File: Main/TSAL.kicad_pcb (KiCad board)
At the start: 2 copper layers, 140 x 70 mm, 81 parts, among them J1 Mini-SPOX, J2 Mini-SPOX, J3 Mini-Fit_Jr, J4 Mini-SPOX, J5 Mini-SPOX, J6 Jumper, J7 Jumper, Q1 IRLML2502, Q2 IRLML2502, Q3 IRLML2502, Q4 IRLML2502, Q5 IRF8721, U1 74HC08, U2 74HC08, U3 TLV70033, U4 LMC555, U5 LMR14030, U6 ZLDO1117G50, U7 TPS62205, U8 MAX40200AUK

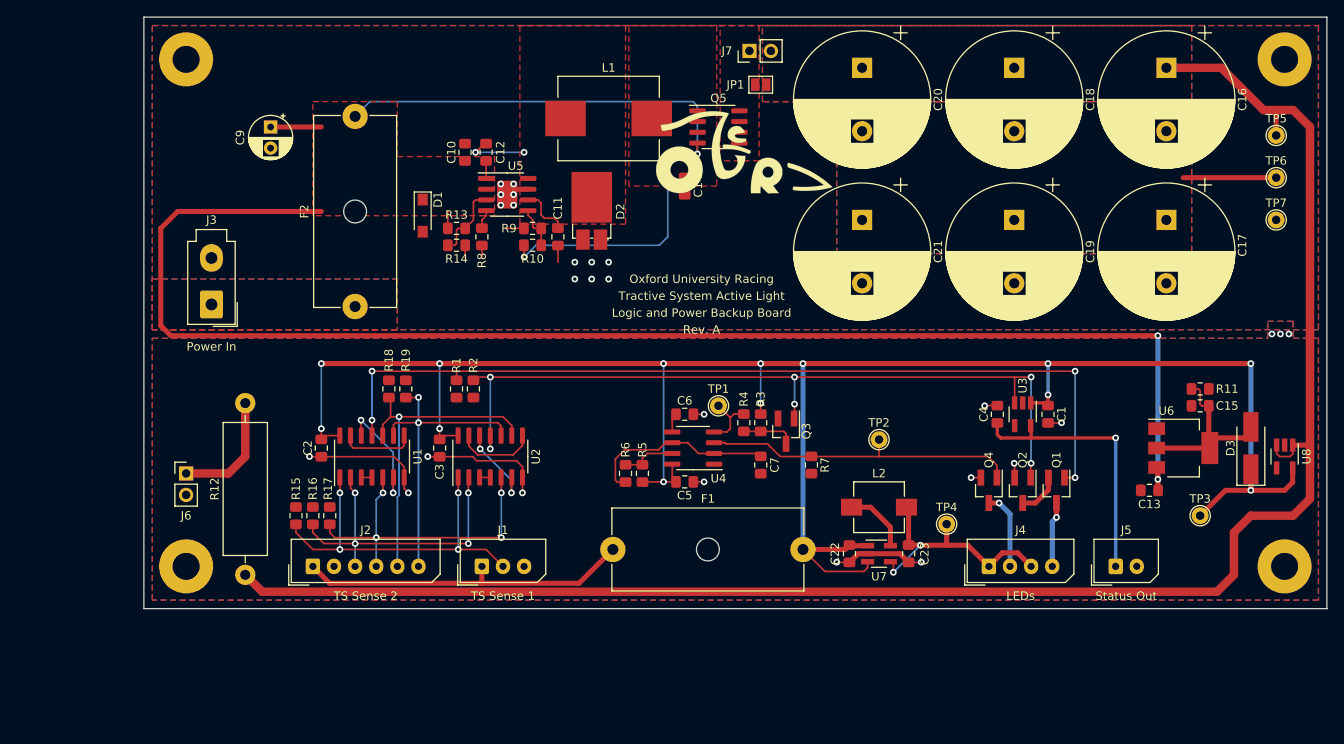
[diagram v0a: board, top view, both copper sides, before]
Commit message: Added first rev of design of new TSAL main board
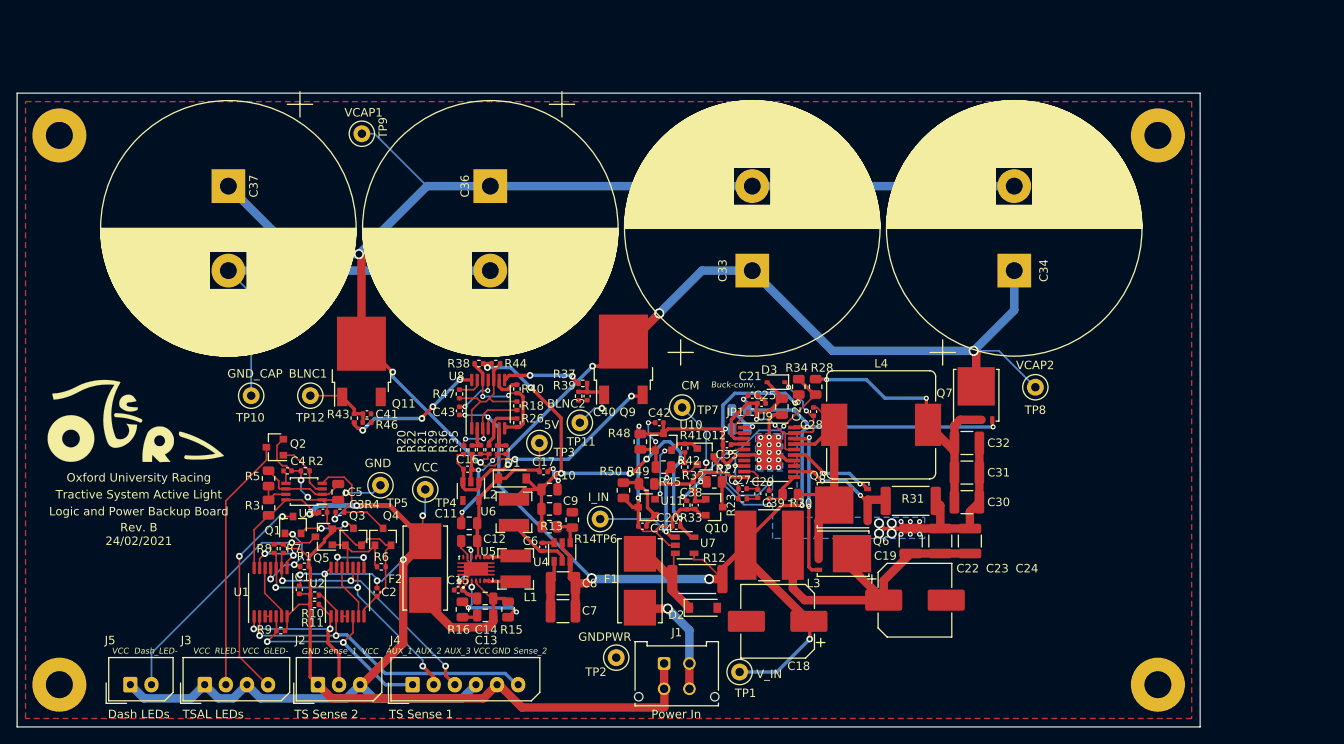
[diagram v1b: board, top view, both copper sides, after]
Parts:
- removed J6, J7: Jumper, Connector_PinHeader_2.54mm:PinHeader_1x02_P2.54mm_Vertical
- added C24: 10uF, Capacitor_SMD:C_1210_3225Metric, F.Cu at (177.8, 122.0)
- added C25: 0.1uF, Capacitor_SMD:C_0402_1005Metric, F.Cu at (153.1, 105.7)
- added C26: 10uF, Capacitor_SMD:C_0805_2012Metric, F.Cu at (155.5, 106.1)
- added C27: 100pF, Capacitor_SMD:C_0402_1005Metric, F.Cu at (150.8, 115.8)
- added C28: 0.1uF, Capacitor_SMD:C_0402_1005Metric, F.Cu at (159.2, 106.7)
- added C29: 1nF, Capacitor_SMD:C_0402_1005Metric, F.Cu at (152.7, 116.4)
- added C30: 100uF, Capacitor_SMD:C_1210_3225Metric, F.Cu at (177.4, 117.4)
- added C31: 100uF, Capacitor_SMD:C_1210_3225Metric, F.Cu at (177.4, 113.9)
- added C32: 100uF, Capacitor_SMD:C_1210_3225Metric, F.Cu at (177.4, 110.4)
- added C33: 200F, Capacitor_THT:CP_Radial_D30.0mm_P10.00mm_SnapIn, F.Cu at (152.0, 90.0)
- added C34: 200F, Capacitor_THT:CP_Radial_D30.0mm_P10.00mm_SnapIn, F.Cu at (183.0, 90.0)
- added C35: 0.1uF, Capacitor_SMD:C_0402_1005Metric, F.Cu at (149.0, 110.6)
- added C36: 200F, Capacitor_THT:CP_Radial_D30.0mm_P10.00mm_SnapIn, F.Cu at (121.0, 80.0)
- added C37: 200F, Capacitor_THT:CP_Radial_D30.0mm_P10.00mm_SnapIn, F.Cu at (90.0, 80.0)
- added C38: 0.1uF, Capacitor_SMD:C_0402_1005Metric, F.Cu at (145.2, 117.8)
- added C39: 1nF, Capacitor_SMD:C_0402_1005Metric, F.Cu at (154.0, 116.5)
- added C40: 0.1uF, Capacitor_SMD:C_0402_1005Metric, F.Cu at (132.4, 104.8)
- added C41: 0.1uF, Capacitor_SMD:C_0402_1005Metric, F.Cu at (106.4, 107.0)
- added C42: 1nF, Capacitor_SMD:C_0402_1005Metric, F.Cu at (141.0, 108.0)
- added C43: 0.1uF, Capacitor_SMD:C_0402_1005Metric, F.Cu at (117.3, 106.6)
- added C44: 1nF, Capacitor_SMD:C_0402_1005Metric, F.Cu at (139.0, 120.2)
- added C8: 10uF, Capacitor_SMD:C_1210_3225Metric, F.Cu at (129.6, 127.0)
- added L3: 2.2uH, Inductor_SMD:L_Bourns-SRN8040_8x8.15mm, F.Cu at (154.0, 122.5)
- added L4: 3.3uH, Inductor_SMD:L_Bourns_SRP1245A, F.Cu at (167.2, 108.2)
- added Q10: NPN, Package_TO_SOT_SMD:SOT-23, F.Cu at (147.5, 118.0)
- added Q11: MJD122, Package_TO_SOT_SMD:TO-252-2, F.Cu at (105.8, 100.8)
- added Q12: PNP, Package_TO_SOT_SMD:SOT-23, F.Cu at (146.5, 112.0)
- added Q6: BSC0904NSI, Package_TO_SOT_SMD:TDSON-8-1, F.Cu at (162.8, 123.5)
- added Q7: BSC0902NSI, Package_TO_SOT_SMD:TDSON-8-1, F.Cu at (178.5, 104.8)
- added Q8: BSC0902NSI, Package_TO_SOT_SMD:TDSON-8-1, F.Cu at (162.8, 117.8)
- added Q9: MJD122, Package_TO_SOT_SMD:TO-252-2, F.Cu at (136.8, 100.5)
- added R20: 10k, Resistor_SMD:R_0402_1005Metric, F.Cu at (117.8, 111.2)
- added R21: 10k, Resistor_SMD:R_0402_1005Metric, F.Cu at (119.8, 111.2)
- added R22: 10k, Resistor_SMD:R_0402_1005Metric, F.Cu at (118.8, 111.2)
- added R23: 47k, Resistor_SMD:R_0402_1005Metric, F.Cu at (150.8, 117.0)
- added R24: 0, project:Trace_0.4mmx0.8mm, F.Cu at (158.0, 109.9)
- added R25: 0, project:Trace_0.4mmx0.8mm, F.Cu at (158.0, 111.8)
- added R26: 10k, Resistor_SMD:R_0402_1005Metric, F.Cu at (124.2, 108.0)
- added R27: 15k, Resistor_SMD:R_0805_2012Metric, F.Cu at (147.5, 115.0)
- added R28: 68k, Resistor_SMD:R_0805_2012Metric, F.Cu at (159.5, 103.8)
- added R29: 10k, Resistor_SMD:R_0402_1005Metric, F.Cu at (120.8, 111.2)
- added R30: 56k, Resistor_SMD:R_0805_2012Metric, F.Cu at (156.5, 116.5)
- added R31: 0.006, Resistor_SMD:R_2512_6332Metric, F.Cu at (170.8, 117.2)
- added R32: 10k, Resistor_SMD:R_0402_1005Metric, F.Cu at (145.0, 115.5)
- added R33: 47k, Resistor_SMD:R_0402_1005Metric, F.Cu at (144.2, 117.8)
- added R34: 12k, Resistor_SMD:R_0805_2012Metric, F.Cu at (157.5, 103.8)
- added R35: 10k, Resistor_SMD:R_0402_1005Metric, F.Cu at (122.8, 111.2)
- added R36: 10k, Resistor_SMD:R_0402_1005Metric, F.Cu at (121.8, 111.2)
- added R37: 1k, Resistor_SMD:R_0402_1005Metric, F.Cu at (131.9, 103.3)
- added R38: 47k, Resistor_SMD:R_0402_1005Metric, F.Cu at (119.7, 101.0)
- added R39: 100k, Resistor_SMD:R_0402_1005Metric, F.Cu at (131.4, 104.8)
- added R40: 1k, Resistor_SMD:R_0402_1005Metric, F.Cu at (124.2, 104.0)
- added R41: 10k, Resistor_SMD:R_0402_1005Metric, F.Cu at (144.0, 111.0)
- added R42: 1k, Resistor_SMD:R_0402_1005Metric, F.Cu at (144.0, 113.2)
- added R43: 1k, Resistor_SMD:R_0402_1005Metric, F.Cu at (104.9, 107.5)
- added R44: 47k, Resistor_SMD:R_0402_1005Metric, F.Cu at (121.7, 101.0)
- added R45: 15k, Resistor_SMD:R_0805_2012Metric, F.Cu at (141.5, 113.2)
- added R46: 100k, Resistor_SMD:R_0402_1005Metric, F.Cu at (106.4, 108.0)
- added R47: 1k, Resistor_SMD:R_0402_1005Metric, F.Cu at (117.3, 104.6)
- added R48: 10k, Resistor_SMD:R_0805_2012Metric, F.Cu at (138.8, 110.2)
- added R49: 10k, Resistor_SMD:R_0805_2012Metric, F.Cu at (139.5, 115.2)
- added R50: 15k, Resistor_SMD:R_0805_2012Metric, F.Cu at (136.8, 116.0)
- added TP10: ~, TestPoint:TestPoint_Loop_D2.50mm_Drill1.0mm, F.Cu at (92.7, 104.8)
- added TP11: ~, TestPoint:TestPoint_Loop_D2.50mm_Drill1.0mm, F.Cu at (131.6, 108.0)
- added TP12: ~, TestPoint:TestPoint_Loop_D2.50mm_Drill1.0mm, F.Cu at (99.7, 104.8)
- added TP8: ~, TestPoint:TestPoint_Loop_D2.50mm_Drill1.0mm, F.Cu at (185.5, 103.8)
- added TP9: ~, TestPoint:TestPoint_Loop_D2.50mm_Drill1.0mm, F.Cu at (105.8, 73.8)
- added U10: TLV431, Package_TO_SOT_SMD:SOT-23, F.Cu at (141.5, 110.2)
- added U11: TLV431, Package_TO_SOT_SMD:SOT-23, F.Cu at (139.5, 118.0)
- added U9: LM25117, Package_SO:ETSSOP-20-1EP_4.4x6.5mm_P0.65mm_EP3x4.2mm, F.Cu at (154.0, 111.5)
- added ZZ1: ~, project:Trace_0.2mmx0.6mm, F.Cu at (142.7, 123.9)
- added ZZ2: ~, project:Trace_0.2mmx0.6mm, F.Cu at (145.1, 124.0)
- added ZZ3: ~, project:Trace_1mmx2mm, F.Cu at (141.6, 140.9)
- added ZZ4: ~, project:Trace_0.2mmx0.6mm, F.Cu at (117.3, 111.8)
- added ZZ5: ~, project:Trace_0.2mmx0.6mm, F.Cu at (157.8, 113.8)
- added ZZ6: ~, project:Trace_0.2mmx0.6mm, F.Cu at (120.7, 112.1)
- added ZZ7: ~, project:Trace_0.2mmx0.6mm, F.Cu at (157.0, 112.8)
- added ZZ8: ~, project:Trace_0.4mmx0.8mm, F.Cu at (152.0, 111.8)
- added ZZ9: ~, project:Trace_0.2mmx0.6mm, F.Cu at (122.3, 111.7)
- C1, C15, C4: value 10u -> 0.1uF; footprint Capacitor_SMD:C_0805_2012Metric_Pad1.15x1.40mm_HandSolder -> Capacitor_SMD:C_0402_1005Metric
- C10, C13, C14: value 10u -> 10uF; footprint Capacitor_SMD:C_0805_2012Metric_Pad1.15x1.40mm_HandSolder -> Capacitor_SMD:C_0805_2012Metric
- C11, C12: value 100n -> 10uF; footprint Capacitor_SMD:C_0805_2012Metric_Pad1.15x1.40mm_HandSolder -> Capacitor_SMD:C_0805_2012Metric
- C16, C17: value 35 -> 0.1uF; footprint Capacitor_THT:CP_Radial_D16.0mm_P7.50mm -> Capacitor_SMD:C_0402_1005Metric
- C18, C19: value 35 -> 220uF; footprint Capacitor_THT:CP_Radial_D16.0mm_P7.50mm -> Capacitor_SMD:CP_Elec_8x10.5
- C2, C3, C6: value 100n -> 0.1uF; footprint Capacitor_SMD:C_0805_2012Metric_Pad1.15x1.40mm_HandSolder -> Capacitor_SMD:C_0402_1005Metric
- C20, C21: value DNP -> 0.1uF; footprint Capacitor_THT:CP_Radial_D16.0mm_P7.50mm -> Capacitor_SMD:C_0402_1005Metric
- C22, C23: value 10u -> 10uF; footprint Capacitor_SMD:C_0805_2012Metric_Pad1.15x1.40mm_HandSolder -> Capacitor_SMD:C_1210_3225Metric
- C5: value 100n -> 2.2uF; footprint Capacitor_SMD:C_0805_2012Metric_Pad1.15x1.40mm_HandSolder -> Capacitor_SMD:C_0805_2012Metric
- C7: value 2.2u -> 10uF; footprint Capacitor_SMD:C_0805_2012Metric_Pad1.15x1.40mm_HandSolder -> Capacitor_SMD:C_1210_3225Metric
- C9: value 100u -> 10uF; footprint Capacitor_THT:CP_Radial_D5.0mm_P2.50mm -> Capacitor_SMD:C_0805_2012Metric
- D1: value SMF4L15A -> ~; footprint project:D_SOD-123_HandSolder -> Diode_SMD:D_SOD-123
- D2: value FSV1045V -> SMF4L15A; footprint project:TO-277A_HandSolder -> Diode_SMD:D_SOD-123
- D3: value S1A -> ~; footprint Diode_SMD:D_SMA_Handsoldering -> Diode_SMD:D_SOD-323
- F1: value 1A -> 6A; footprint Fuse:Fuseholder_Cylinder-5x20mm_Schurter_0031_8201_Horizontal_Open -> footprints_archive_old_design:Fuseholder_Littelfuse_Nano2_154x
- F2: value 3A -> 1A; footprint Fuse:Fuseholder_Cylinder-5x20mm_Schurter_0031_8201_Horizontal_Open -> footprints_archive_old_design:Fuseholder_Littelfuse_Nano2_154x
- J1: value Mini-SPOX -> Micro-Fit; footprint Connector_Molex:Molex_SPOX_5267-03A_1x03_P2.50mm_Vertical -> Connector_Molex:Molex_Micro-Fit_3.0_43045-0412_2x02_P3.00mm_Vertical
- J2: footprint Connector_Molex:Molex_SPOX_5267-06A_1x06_P2.50mm_Vertical -> Connector_Molex:Molex_SPOX_5267-03A_1x03_P2.50mm_Vertical
- J3: value Mini-Fit_Jr -> Mini-SPOX; footprint Connector_Molex:Molex_Mini-Fit_Jr_5566-02A_2x01_P4.20mm_Vertical -> Connector_Molex:Molex_SPOX_5267-04A_1x04_P2.50mm_Vertical
- J4: footprint Connector_Molex:Molex_SPOX_5267-04A_1x04_P2.50mm_Vertical -> Connector_Molex:Molex_SPOX_5267-06A_1x06_P2.50mm_Vertical
- JP1: value Jumper -> 0; footprint Jumper:SolderJumper-2_P1.3mm_Open_Pad1.0x1.5mm -> Resistor_SMD:R_0402_1005Metric
- L1: value 15u -> 1.5uH; footprint project:104CDMCCDS -> Inductor_SMD:L_Bourns-SRN4018
- L2: value 10u -> 4.7uH; footprint project:CDRH62B -> Inductor_SMD:L_Bourns-SRN4018
- Q1, Q2, Q3, Q4: footprint Package_TO_SOT_SMD:SOT-23_Handsoldering -> Package_TO_SOT_SMD:SOT-23
- Q5: value IRF8721 -> IRLML2502; footprint Package_SO:SOIC-8_3.9x4.9mm_P1.27mm -> Package_TO_SOT_SMD:SOT-23
- R1, R2, R6, R7, R8: footprint Resistor_SMD:R_0805_2012Metric_Pad1.15x1.40mm_HandSolder -> Resistor_SMD:R_0402_1005Metric
- R10: value 130k -> 100k; footprint Resistor_SMD:R_0805_2012Metric_Pad1.15x1.40mm_HandSolder -> Resistor_SMD:R_0402_1005Metric
- R11: value 1k -> 100k; footprint Resistor_SMD:R_0805_2012Metric_Pad1.15x1.40mm_HandSolder -> Resistor_SMD:R_0402_1005Metric
- R12: value 4.7 -> 0.006; footprint Resistor_THT:R_Axial_DIN0516_L15.5mm_D5.0mm_P20.32mm_Horizontal -> Resistor_SMD:R_2512_6332Metric
- R13: value 820k -> 56k; footprint Resistor_SMD:R_0805_2012Metric_Pad1.15x1.40mm_HandSolder -> Resistor_SMD:R_0805_2012Metric
- R14, R16: value 100k -> 10k; footprint Resistor_SMD:R_0805_2012Metric_Pad1.15x1.40mm_HandSolder -> Resistor_SMD:R_0805_2012Metric
- R15: value 100k -> 56k; footprint Resistor_SMD:R_0805_2012Metric_Pad1.15x1.40mm_HandSolder -> Resistor_SMD:R_0805_2012Metric
- R17: value 100k -> 68k; footprint Resistor_SMD:R_0805_2012Metric_Pad1.15x1.40mm_HandSolder -> Resistor_SMD:R_0805_2012Metric; moved to B.Cu
- R18: value 100k -> 10k; footprint Resistor_SMD:R_0805_2012Metric_Pad1.15x1.40mm_HandSolder -> Resistor_SMD:R_0402_1005Metric
- R19: value 100k -> 10k; footprint Resistor_SMD:R_0805_2012Metric_Pad1.15x1.40mm_HandSolder -> Resistor_SMD:R_0805_2012Metric; moved to B.Cu
- R3: value 22k -> 10k; footprint Resistor_SMD:R_0805_2012Metric_Pad1.15x1.40mm_HandSolder -> Resistor_SMD:R_0805_2012Metric
- R4: value 1k -> 10k; footprint Resistor_SMD:R_0805_2012Metric_Pad1.15x1.40mm_HandSolder -> Resistor_SMD:R_0402_1005Metric
- R5: value 22k -> 100k; footprint Resistor_SMD:R_0805_2012Metric_Pad1.15x1.40mm_HandSolder -> Resistor_SMD:R_0805_2012Metric
- R9: value 22k -> 100k; footprint Resistor_SMD:R_0805_2012Metric_Pad1.15x1.40mm_HandSolder -> Resistor_SMD:R_0402_1005Metric
- TP1: value TP_Timer_En -> ~; footprint TestPoint:TestPoint_THTPad_D2.0mm_Drill1.0mm -> TestPoint:TestPoint_Loop_D2.50mm_Drill1.0mm
- TP2: value TP_RLED_Ctrl -> ~; footprint TestPoint:TestPoint_THTPad_D2.0mm_Drill1.0mm -> TestPoint:TestPoint_Loop_D2.50mm_Drill1.0mm
- TP3: value TP_VCC -> ~; footprint TestPoint:TestPoint_THTPad_D2.0mm_Drill1.0mm -> TestPoint:TestPoint_Loop_D2.50mm_Drill1.0mm
- TP4: value TP_2V5 -> ~; footprint TestPoint:TestPoint_THTPad_D2.0mm_Drill1.0mm -> TestPoint:TestPoint_Loop_D2.50mm_Drill1.0mm
- TP5: value TP_Vcap -> ~; footprint TestPoint:TestPoint_THTPad_D2.0mm_Drill1.0mm -> TestPoint:TestPoint_Loop_D2.50mm_Drill1.0mm
- TP6: value TP_Vmid -> ~; footprint TestPoint:TestPoint_THTPad_D2.0mm_Drill1.0mm -> TestPoint:TestPoint_Loop_D2.50mm_Drill1.0mm
- TP7: value TP_GND -> ~; footprint TestPoint:TestPoint_THTPad_D2.0mm_Drill1.0mm -> TestPoint:TestPoint_Loop_D2.50mm_Drill1.0mm
- U1, U2: footprint Package_SO:SOIC-14_3.9x8.7mm_P1.27mm -> Package_SO:TSSOP-14_4.4x5mm_P0.65mm
- U3: value TLV70033 -> LMC555; footprint Package_TO_SOT_SMD:SOT-23-5_HandSoldering -> Package_SO:TSSOP-8_3x3mm_P0.65mm
- U4: value LMC555 -> TPS562200; footprint Package_SO:SOIC-8_3.9x4.9mm_P1.27mm -> Package_TO_SOT_SMD:SOT-23-6
- U5: value LMR14030 -> TPS63020; footprint Package_SO:SOIC-8-1EP_3.9x4.9mm_P1.27mm_EP2.41x3.3mm -> project:TPS63020
- U6: value ZLDO1117G50 -> MAX40200AUK; footprint Package_TO_SOT_SMD:SOT-223-3_TabPin2 -> Package_TO_SOT_SMD:SOT-23-5
- U7: value TPS62205 -> INA180A3; footprint Package_TO_SOT_SMD:SOT-23-5_HandSoldering -> Package_TO_SOT_SMD:SOT-23-5
- U8: value MAX40200AUK -> TLV9104; footprint Package_TO_SOT_SMD:SOT-23-5_HandSoldering -> Package_SO:TSSOP-14_4.4x5mm_P0.65mm
- moved J5 117.4 mm to (78.4, 139.0)
- moved TP5 113.8 mm to (108.0, 115.4), turned to 90 degrees
- moved R11 107.9 mm to (100.2, 129.5), turned to 180 degrees
- moved C16 95.4 mm to (118.3, 113.5), turned to 0 degrees
- moved U8 94.5 mm to (120.8, 105.8), turned to 90 degrees
- moved C1 91.0 mm to (98.4, 127.8)
- moved C15 90.5 mm to (117.2, 127.8), turned to 0 degrees
- moved Q1 90.4 mm to (97.7, 120.1), turned to 90 degrees
- moved TP6 89.6 mm to (134.0, 119.4), turned to 90 degrees
- moved Q2 88.6 mm to (95.5, 110.9), turned to 180 degrees
- moved U3 85.5 mm to (99.0, 116.1), turned to 180 degrees
- moved U6 84.5 mm to (118.7, 116.1), turned to 270 degrees
- moved C4 84.3 mm to (97.0, 113.7), turned to 0 degrees
- moved C13 80.0 mm to (120.4, 130.8)
- moved C17 79.5 mm to (127.3, 113.8), turned to 0 degrees
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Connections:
- C10 pad 1: /Power/VIN_F -> +5V
- C10 pad 2: GND -> GNDPWR
- C11 pad 2: GND -> GNDPWR
- C12 pad 1: Net-(C12-Pad1) -> Net-(C11-Pad1)
- C12 pad 2: Net-(C12-Pad2) -> GNDPWR
- C13 pad 1: /Power/VIN_F -> Net-(C13-Pad1)
- C13 pad 2: GND -> GNDPWR
- C14 pad 1: Net-(C14-Pad1) -> Net-(C13-Pad1)
- C14 pad 2: GND -> GNDPWR
- C15 pad 2: GND -> GNDPWR
- C16 pad 1: /Power/Vcap -> /Power/VCAP2
- C16 pad 2: Net-(C16-Pad2) -> GNDPWR
- C17 pad 1: Net-(C16-Pad2) -> Net-(C11-Pad1)
- C17 pad 2: GND -> GNDPWR
- C18 pad 1: /Power/Vcap -> /Power/V_IN
- C18 pad 2: Net-(C16-Pad2) -> GNDPWR
- C19 pad 1: Net-(C16-Pad2) -> Net-(C19-Pad1)
- C19 pad 2: GND -> GNDPWR
- C20 pad 1: /Power/Vcap -> +5V
- C20 pad 2: Net-(C16-Pad2) -> GNDA
- C21 pad 1: Net-(C16-Pad2) -> /Power/V_IN
- C21 pad 2: GND -> GNDPWR
- C22 pad 1: VCC -> Net-(C19-Pad1)
- C22 pad 2: GND -> GNDPWR
- C23 pad 1: +2V5 -> Net-(C19-Pad1)
- C23 pad 2: GND -> GNDPWR
- C4 pad 1: /TS_Inact_Out -> Net-(C4-Pad1)
- C5 pad 1: VCC -> Net-(C5-Pad1)
- C6 pad 2: GND -> Net-(C6-Pad2)
- C7 pad 1: Net-(C7-Pad1) -> /Power/V_IN
- C7 pad 2: GND -> GNDPWR
- C9 pad 1: /Power/VIN_F -> +5V
- C9 pad 2: GND -> GNDPWR
- D1 pad 1: /Power/VIN_F -> Net-(C11-Pad1)
- D1 pad 2: GND -> +5V
- D2 pad 1: GND -> Net-(D2-Pad1)
- D2 pad 2: GND -> GNDPWR
- D3 pad 1: VCC -> /Power/HB
- D3 pad 2: Net-(C15-Pad1) -> /Power/BUCK_VCC
- F1 pad 1: /VCC_F -> Net-(D2-Pad1)
- F1 pad 2: VCC -> VIN
- F2 pad 1: /Power/VIN_F -> VCC
- F2 pad 2: VIN -> Net-(C13-Pad1)
- J1 pad 1: /VCC_F -> GNDPWR
- J1 pad 2: /Sense_1 -> VIN
- J1 pad 3: GND -> GNDPWR
- J2 pad 1: /VCC_F -> GND
- J2 pad 2: GND -> /Sense_1
- J2 pad 3: /Sense_2 -> VCC
- J3 pad 1: VIN -> VCC
- J3 pad 2: GND -> /RLED-
- J4 pad 1: +2V5 -> /AUX_1
- J4 pad 2: /RLED- -> /AUX_2
- J4 pad 3: +2V5 -> /AUX_3
- J4 pad 4: /GLED- -> VCC
- J5 pad 1: /TS_Inact_Out -> VCC
- J5 pad 2: GND -> /Dash_LED-
- JP1 pad 1: Net-(J7-Pad1) -> /Power/BUCK_VCC
- JP1 pad 2: /Power/Vcap -> /Power/DEMB
- L1 pad 1: Net-(C12-Pad2) -> Net-(L1-Pad1)
- L1 pad 2: Net-(C14-Pad1) -> Net-(L1-Pad2)
- L2 pad 1: Net-(L2-Pad1) -> Net-(C6-Pad1)
- L2 pad 2: +2V5 -> +5V
- Q2 pad 3: Net-(Q1-Pad2) -> /RLED-
- Q3 pad 1: Net-(Q2-Pad1) -> Net-(Q3-Pad1)
- Q3 pad 3: Net-(Q3-Pad3) -> Net-(Q1-Pad2)
- Q4 pad 1: Net-(Q4-Pad1) -> Net-(Q3-Pad1)
- Q4 pad 3: /RLED- -> Net-(Q4-Pad3)
- Q5 pad 1: Net-(C14-Pad1) -> Net-(Q3-Pad1)
- Q5 pad 2: Net-(C14-Pad1) -> GND
- Q5 pad 3: Net-(C14-Pad1) -> /Dash_LED-
- R10 pad 1: Net-(C14-Pad1) -> /Sense_2
- R10 pad 2: Net-(R10-Pad2) -> GND
- R11 pad 1: Net-(C15-Pad1) -> /Sense_1
- R12 pad 1: /Power/Vcap -> Net-(D2-Pad1)
- R12 pad 2: Net-(J6-Pad1) -> /Power/V_IN
- R13 pad 1: /Power/VIN_F -> +5V
- R14 pad 2: GND -> GNDPWR
- R15 pad 1: /Sense_1 -> Net-(C13-Pad1)
- R15 pad 2: GND -> Net-(R15-Pad2)
- R16 pad 1: /Sense_2 -> Net-(R15-Pad2)
- R16 pad 2: GND -> GNDPWR
- R17 pad 1: /AUX_1 -> /Power/V_IN
- R17 pad 2: GND -> /Power/UVLO
- R18 pad 1: /AUX_2 -> Net-(R18-Pad1)
- R18 pad 2: GND -> /Power/CAP_D2
- R19 pad 1: /AUX_3 -> /Power/UVLO
- R19 pad 2: GND -> GNDA
- R3 pad 2: Net-(Q3-Pad3) -> Net-(R3-Pad2)
- R4 pad 1: Net-(R4-Pad1) -> VCC
- R4 pad 2: Net-(Q3-Pad3) -> Net-(Q4-Pad3)
- R5 pad 1: VCC -> Net-(R3-Pad2)
- R5 pad 2: Net-(R5-Pad2) -> Net-(C5-Pad1)
- R6 pad 1: Net-(R5-Pad2) -> Net-(Q3-Pad1)
- R6 pad 2: Net-(C7-Pad1) -> GND
- R7 pad 1: Net-(Q4-Pad1) -> /AUX_3
- R8 pad 1: Net-(R8-Pad1) -> /AUX_2
- R9 pad 1: Net-(R10-Pad2) -> /AUX_1
- TP1 pad 1: Net-(R4-Pad1) -> /Power/V_IN
- TP2 pad 1: Net-(Q4-Pad1) -> GNDPWR
- TP3 pad 1: VCC -> Net-(C11-Pad1)
- TP4 pad 1: +2V5 -> VCC
- TP5 pad 1: /Power/Vcap -> GND
- TP6 pad 1: Net-(C16-Pad2) -> /Power/I_SENSE
- TP7 pad 1: GND -> /Power/CM
- U2 pad 11: Net-(Q2-Pad1) -> Net-(Q3-Pad1)
- U3 pad 1: VCC -> GND
- U3 pad 2: GND -> Net-(C5-Pad1)
- U3 pad 4: (no net) -> Net-(Q4-Pad3)
- U3 pad 5: /TS_Inact_Out -> Net-(C4-Pad1)
- U4 pad 1: GND -> GNDPWR
- U4 pad 2: Net-(C7-Pad1) -> Net-(C6-Pad1)
- U4 pad 3: Net-(Q4-Pad1) -> /Power/V_IN
- U4 pad 4: Net-(R4-Pad1) -> Net-(R13-Pad2)
- U4 pad 5: Net-(C6-Pad1) -> /Power/V_IN
- U4 pad 6: Net-(C7-Pad1) -> Net-(C6-Pad2)
- U5 pad 1: Net-(C12-Pad1) -> Net-(C15-Pad1)
- U5 pad 2: /Power/VIN_F -> GNDPWR
- U5 pad 3: Net-(R13-Pad2) -> Net-(R15-Pad2)
- U5 pad 4: Net-(R8-Pad1) -> Net-(C13-Pad1)
- U5 pad 5: Net-(R10-Pad2) -> (no net)
- U5 pad 6: Net-(C11-Pad1) -> Net-(L1-Pad2)
- U5 pad 7: GND -> Net-(L1-Pad2)
- U5 pad 8: Net-(C12-Pad2) -> Net-(L1-Pad1)
- U5 pad 9: GND -> Net-(L1-Pad1)
- U6 pad 1: GND -> /Power/VCAP2
- U6 pad 2: Net-(C15-Pad1) -> GNDPWR
- U6 pad 3: /Power/VIN_F -> /Power/VCAP2
- U7 pad 1: VCC -> /Power/I_SENSE
- U7 pad 2: GND -> GNDA
- U7 pad 3: VCC -> /Power/IN_CS+
- U7 pad 4: +2V5 -> /Power/IN_CS-
- U7 pad 5: Net-(L2-Pad1) -> +5V
- U8 pad 1: /Power/Vcap -> /Power/CAP_D2
- U8 pad 2: GND -> Net-(R21-Pad2)
- U8 pad 3: /Power/Vcap -> Net-(R18-Pad1)
- U8 pad 4: (no net) -> /Power/V_IN
- U8 pad 5: VCC -> Net-(R26-Pad1)
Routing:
- net /Power/VIN_F: track 226.0 -> 0.00 mm, vias 3 -> 0
- net /Power/Vcap: track 207.6 -> 0.00 mm
- net /Power/VCAP1: track 0.00 -> 167.7 mm, vias 0 -> 5
- net /Power/V_IN: track 0.00 -> 143.2 mm, vias 0 -> 9
- net GNDPWR: track 0.00 -> 140.4 mm, vias 0 -> 32
- net VCC: track 237.4 -> 128.9 mm, vias 13 -> 8
- net /Power/VCAP2: track 0.00 -> 105.6 mm, vias 0 -> 4
- net Net-(Q1-Pad1): track 105.7 -> 11.0 mm, vias 4 -> 3
- net Net-(Q2-Pad1): track 96.1 -> 7.06 mm, vias 6 -> 0
- net GNDA: track 0.00 -> 71.7 mm, vias 0 -> 6
- net +5V: track 0.00 -> 63.3 mm, vias 0 -> 7
- net GND: track 59.5 -> 115.9 mm, vias 27 -> 3
- net /VCC_F: track 40.0 -> 0.00 mm
- net Net-(Q4-Pad1): track 38.0 -> 0.00 mm
- net Net-(C19-Pad1): track 0.00 -> 37.3 mm
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- added copper zone on B.Cu, net GNDPWR
- added copper zone on F.Cu, net GNDPWR
- removed copper zone on F.Cu, net /Power/VIN_F
- removed copper zone on B.Cu, net /Power/Vcap
- removed copper zone on F.Cu, net /Power/Vcap
- removed copper zone on B.Cu, net GND
- removed copper zone on F.Cu, net GND
- removed copper zone on F.Cu, net Net-(C12-Pad2)
- removed copper zone on F.Cu, net Net-(C14-Pad1)
- removed copper zone on B.Cu, net Net-(C16-Pad2)
- removed copper zone on F.Cu, net Net-(C16-Pad2)
- removed copper zone on F.Cu, net Net-(J7-Pad1)
- removed copper zone on B.Cu, net VIN
- removed copper zone on F.Cu, net VIN
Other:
- board size 140 x 70 mm -> 140 x 75 mm
- board text added: "5V"
- board text added: "AUX_1"
- board text added: "AUX_2"
- board text added: "AUX_3"
- board text added: "BLNC1"
- board text added: "BLNC2"
- board text added: "Buck-conv."
- board text added: "CM"
- board text added: "Dash LEDs"
- board text added: "Dash_LED-"
- board text added: "GLED-"
- board text added: "GND"
- board text added: "GNDPWR"
- board text added: "GND_CAP"
- board text added: "I_IN"
- board text added: "RLED-"
- board text added: "Rev. B 24/02/2021"
- board text added: "Sense_1"
- board text added: "Sense_2"
- board text added: "TSAL LEDs"
- board text added: "VCAP1"
- board text added: "VCAP2"
- board text added: "VCC"
- board text added: "V_IN"
- board text removed: "LEDs"
- board text removed: "Rev. A"
- board text removed: "Status Out"
